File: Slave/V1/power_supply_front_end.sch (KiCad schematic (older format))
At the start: 13 parts, among them U601 AP3015KTR-G1, U602 AP2202K-ADJTRG1

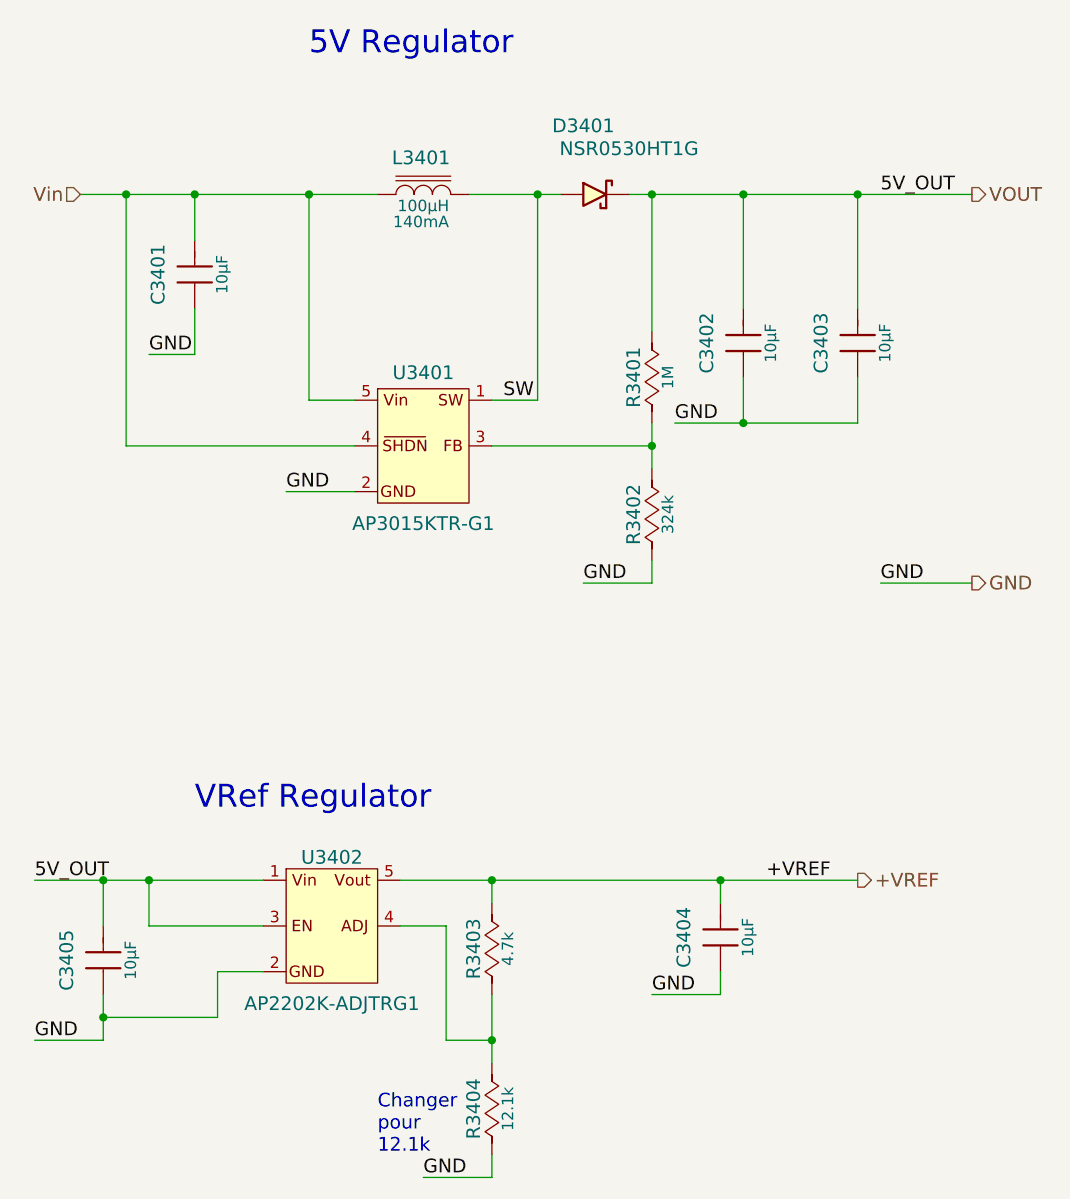
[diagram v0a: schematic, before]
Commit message: Routing signals
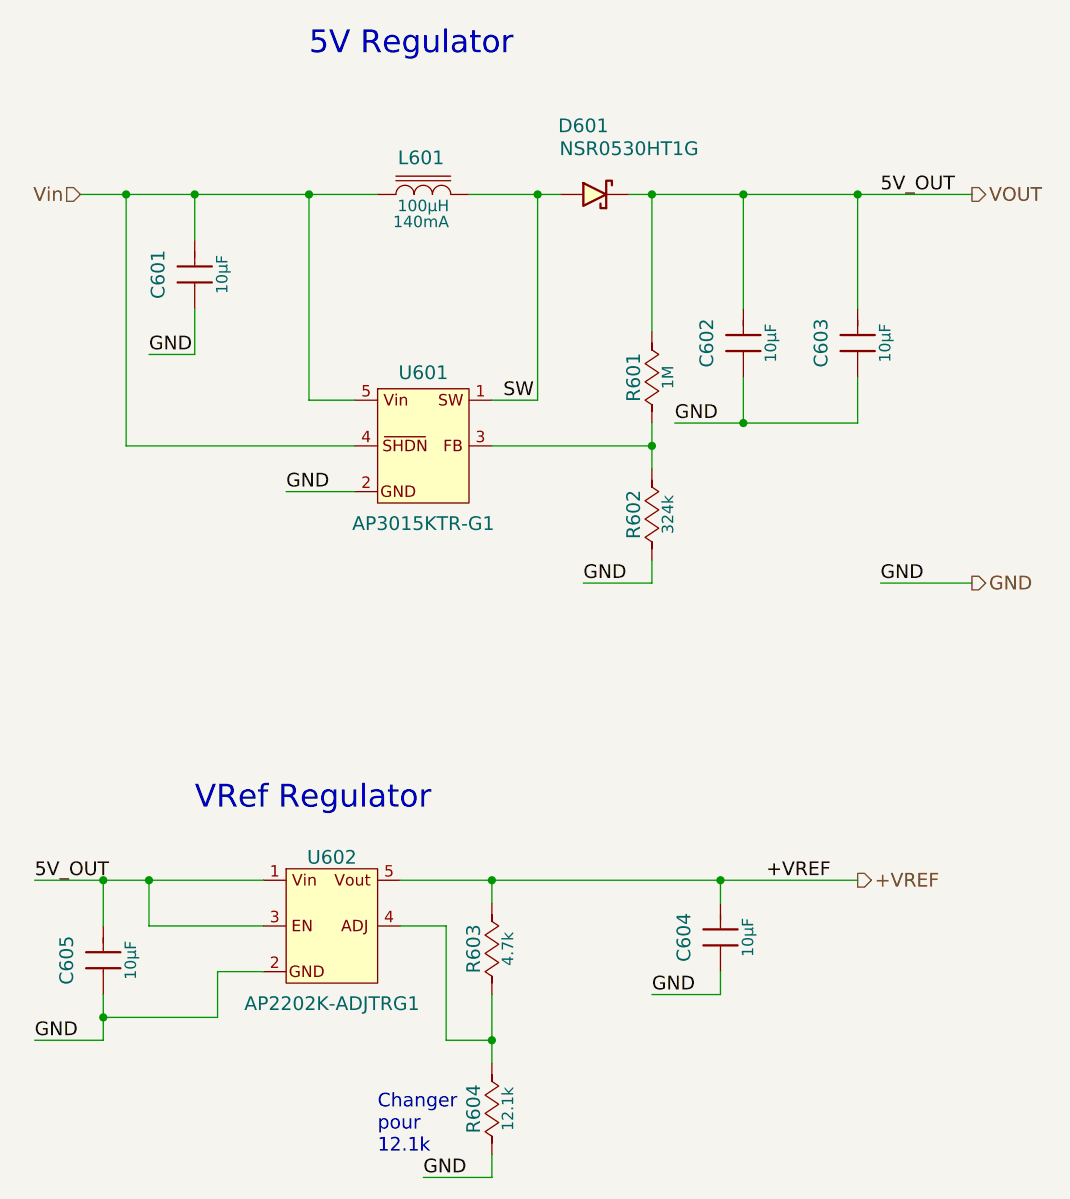
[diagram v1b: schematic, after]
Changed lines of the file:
@@
 AR Path="/59400D56/591CDE38/591B2FEB" Ref="U3001"  Part="1"
 AR Path="/59400D60/591CDE38/591B2FEB" Ref="U3401"  Part="1"
-F 0 "U3401" H 4900 3220 60  0000 C CNN
+F 0 "U601" H 4900 3220 60  0000 C CNN
 F 1 "AP3015KTR-G1" H 4900 2560 60  0000 C CNN
 F 2 "IC:SOT-23-5" H 4900 475 60  0001 C CNN
@@
 AR Path="/59400D56/591CDE38/591B30B0" Ref="U3002"  Part="1"
 AR Path="/59400D60/591CDE38/591B30B0" Ref="U3402"  Part="1"
-F 0 "U3402" H 4500 5300 60  0000 C CNN
+F 0 "U602" H 4500 5300 60  0000 C CNN
 F 1 "AP2202K-ADJTRG1" H 4500 4660 60  0000 C CNN
 F 2 "IC:SOT-23-5" H 4500 3395 60  0001 C CNN
@@
 AR Path="/59400D56/591CDE38/591BCA3D" Ref="C3001"  Part="1"
 AR Path="/59400D60/591CDE38/591BCA3D" Ref="C3401"  Part="1"
-F 0 "C3401" H 3850 2260 60  0000 C CNN
+F 0 "C601" H 3850 2260 60  0000 C CNN
 F 1 "885012107014" H 3850 1750 60  0001 C CNN
 F 2 "Capacitors:C0805" H 3850 1150 60  0001 C CNN
@@
 AR Path="/59400D56/591CDE38/591BD4B8" Ref="D3001"  Part="1"
 AR Path="/59400D60/591CDE38/591BD4B8" Ref="D3401"  Part="1"
-F 0 "D3401" H 5600 2100 60  0000 C CNN
+F 0 "D601" H 5600 2100 60  0000 C CNN
 F 1 "NSR0530HT1G" H 5800 2000 60  0000 C CNN
 F 2 "Diodes:SOD-323" H 5680 800 60  0001 C CNN
@@
 AR Path="/59400D56/591CDE38/591BE5E6" Ref="C3002"  Part="1"
 AR Path="/59400D60/591CDE38/591BE5E6" Ref="C3402"  Part="1"
-F 0 "C3402" H 6250 2560 60  0000 C CNN
+F 0 "C602" H 6250 2560 60  0000 C CNN
 F 1 "885012107014" H 6250 2050 60  0001 C CNN
 F 2 "Capacitors:C0805" H 6250 1450 60  0001 C CNN
@@
 AR Path="/59400D56/591CDE38/591BED58" Ref="C3005"  Part="1"
 AR Path="/59400D60/591CDE38/591BED58" Ref="C3405"  Part="1"
-F 0 "C3405" H 3450 5260 60  0000 C CNN
+F 0 "C605" H 3450 5260 60  0000 C CNN
 F 1 "885012107014" H 3450 4750 60  0001 C CNN
 F 2 "Capacitors:C0805" H 3450 4150 60  0001 C CNN
@@
 AR Path="/59400D56/591CDE38/591BF617" Ref="C3004"  Part="1"
 AR Path="/59400D60/591CDE38/591BF617" Ref="C3404"  Part="1"
-F 0 "C3404" H 6150 5160 60  0000 C CNN
+F 0 "C604" H 6150 5160 60  0000 C CNN
 F 1 "885012107014" H 6150 4650 60  0001 C CNN
 F 2 "Capacitors:C0805" H 6150 4050 60  0001 C CNN
@@
 AR Path="/59400D56/591CDE38/591BFD48" Ref="C3003"  Part="1"
 AR Path="/59400D60/591CDE38/591BFD48" Ref="C3403"  Part="1"
-F 0 "C3403" H 6750 2560 60  0000 C CNN
+F 0 "C603" H 6750 2560 60  0000 C CNN
 F 1 "885012107014" H 6750 2050 60  0001 C CNN
 F 2 "Capacitors:C0805" H 6750 1450 60  0001 C CNN
@@
 AR Path="/59400D56/591CDE38/591C2F0F" Ref="R3001"  Part="1"
 AR Path="/59400D60/591CDE38/591C2F0F" Ref="R3401"  Part="1"
-F 0 "R3401" H 5900 2680 60  0000 C CNN
+F 0 "R601" H 5900 2680 60  0000 C CNN
 F 1 "RC0805JR-071ML" H 5900 2300 50  0001 C CNN
 F 2 "Resistors:R0805" H 5900 1700 30  0001 C CNN
@@
 AR Path="/59400D56/591CDE38/591C3C0D" Ref="R3002"  Part="1"
 AR Path="/59400D60/591CDE38/591C3C0D" Ref="R3402"  Part="1"
-F 0 "R3402" H 5900 3280 60  0000 C CNN
+F 0 "R602" H 5900 3280 60  0000 C CNN
 F 1 "RC0805FR-07324KL" H 5900 2900 50  0001 C CNN
 F 2 "Resistors:R0805" H 5900 2300 30  0001 C CNN
@@
 AR Path="/59400D56/591CDE38/5938E158" Ref="R3003"  Part="1"
 AR Path="/59400D60/591CDE38/5938E158" Ref="R3403"  Part="1"
-F 0 "R3403" H 5200 5180 60  0000 C CNN
+F 0 "R603" H 5200 5180 60  0000 C CNN
 F 1 "RC0805JR-074K7L" H 5200 4800 50  0001 C CNN
 F 2 "Resistors:R0805" H 5200 4200 30  0001 C CNN
@@
 AR Path="/59400D56/591CDE38/593DE9E8" Ref="R3004"  Part="1"
 AR Path="/59400D60/591CDE38/593DE9E8" Ref="R3404"  Part="1"
-F 0 "R3404" H 5200 5880 60  0000 C CNN
+F 0 "R604" H 5200 5880 60  0000 C CNN
 F 1 "RC0805FR-0712K1L" H 5200 5500 50  0001 C CNN
 F 2 "Resistors:R0805" H 5200 4900 30  0001 C CNN
@@
 AR Path="/59400D56/591CDE38/593D0CFC" Ref="L3001"  Part="1"
 AR Path="/59400D60/591CDE38/593D0CFC" Ref="L3401"  Part="1"
-F 0 "L3401" H 4890 1960 60  0000 C CNN
+F 0 "L601" H 4890 1960 60  0000 C CNN
 F 1 "MLZ2012N101LT000" H 4900 1500 60  0001 C CNN
 F 2 "Inductors:I0805" H 4900 900 60  0001 C CNN

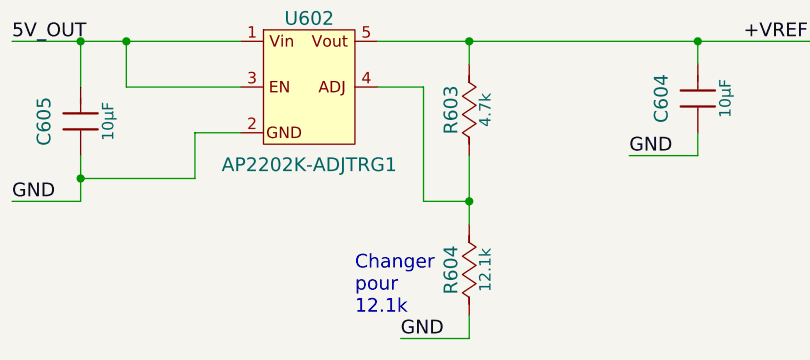
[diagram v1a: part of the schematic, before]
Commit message: minor
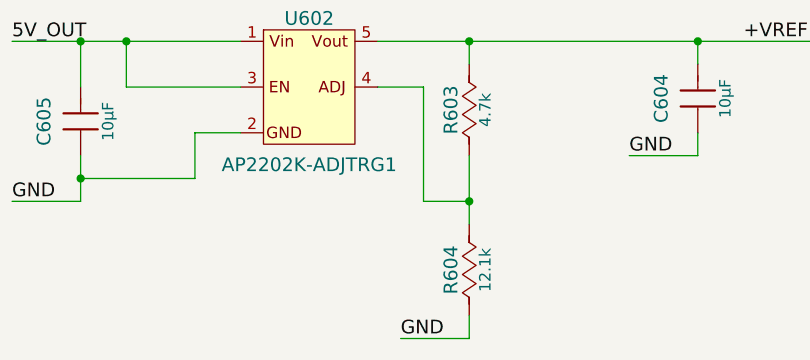
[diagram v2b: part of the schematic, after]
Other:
- note removed: "Changer\npour\n12.1k"
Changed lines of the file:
@@
 $Descr USLetter 11000 8500
 encoding utf-8
-Sheet 14 36
+Sheet 6 36
 Title "Isolated BMS Slave Front End"
 Date ""
@@
 Text HLabel 3400 1800 0    60   Input ~ 0
 Vin
-Text Notes 4700 6000 0    60   ~ 0
-Changer\npour\n12.1k
 Wire Wire Line
 	4600 2900 3600 2900
